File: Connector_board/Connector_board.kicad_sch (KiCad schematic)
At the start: 6 parts, among them J1 USB_B_Micro, J2 Conn_02x04_Counter_Clockwise, J3 Conn_02x06_Counter_Clockwise, J4 Conn_02x07_Counter_Clockwise

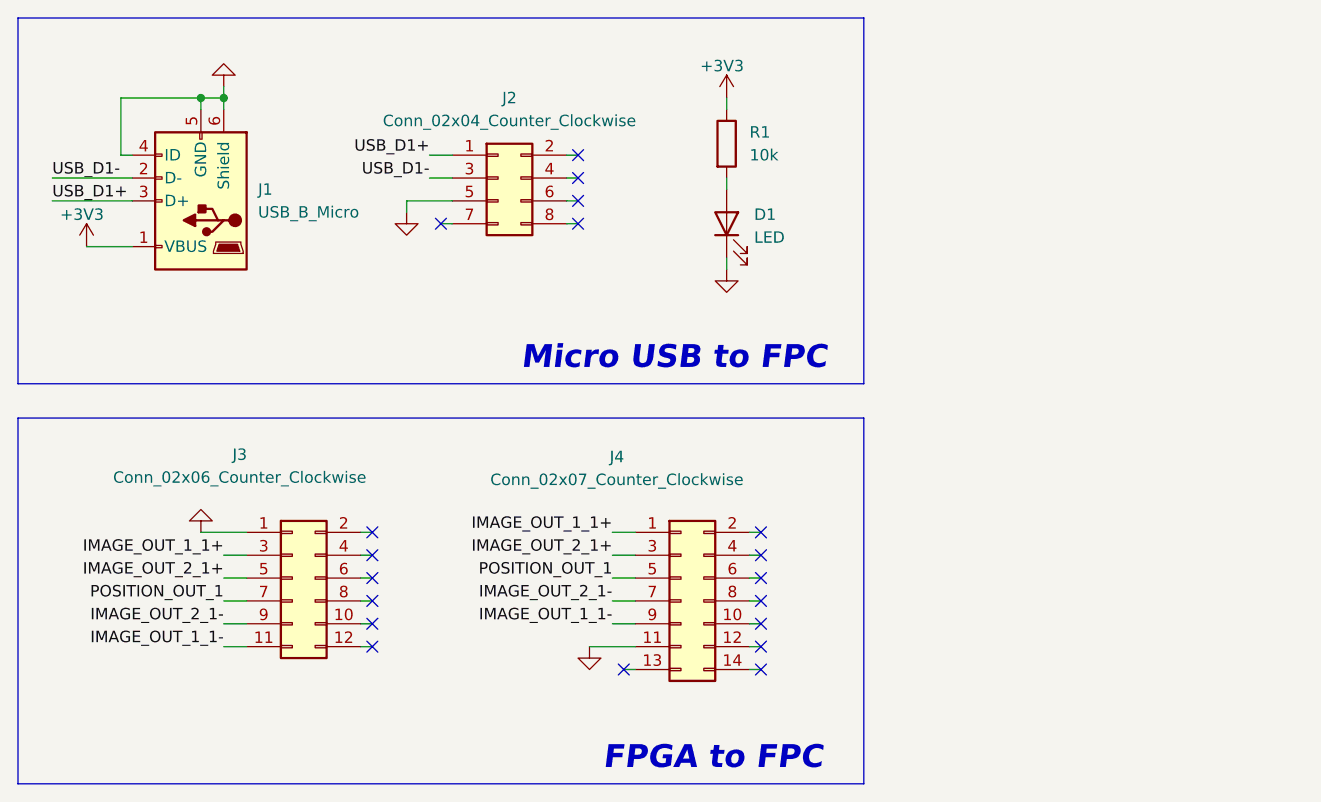
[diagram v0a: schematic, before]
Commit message: layout finalized (?)
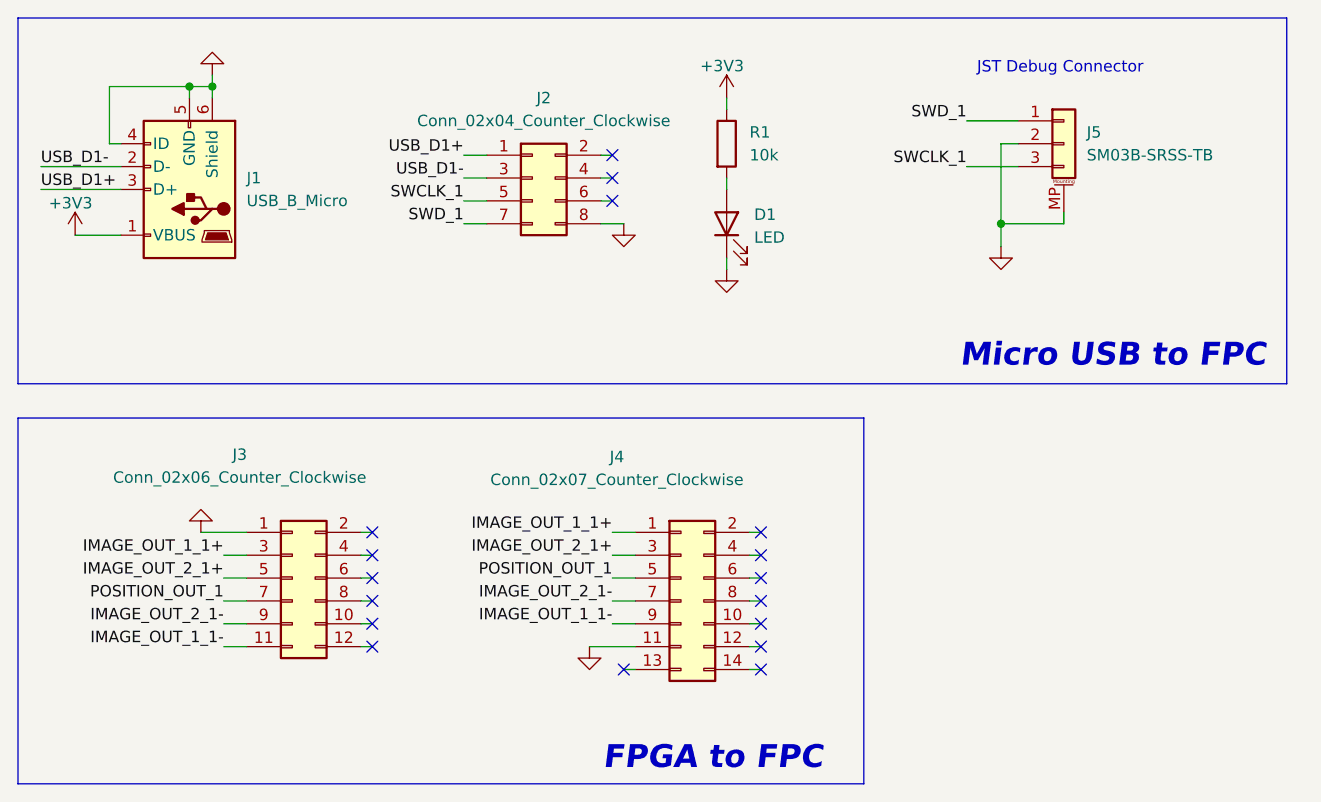
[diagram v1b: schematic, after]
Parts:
- added J5: SM03B-SRSS-TB, Connector_JST:JST_SH_SM03B-SRSS-TB_1x03-1MP_P1.00mm_Horizontal, symbol Connector_Generic_MountingPin:Conn_01x03_MountingPin
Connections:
- net GND: now also J2.8 (Pin_8), J5.2 (Pin_2), J5.MP (MountPin); no longer J2.5 (Pin_5)
- net SWD_1: now reaches J2.7 (Pin_7)
- net SWD_1: now also J5.1 (Pin_1)
- new net SWCLK_1: J2.5 (Pin_5), J5.3 (Pin_3)
- no-connect marks 19 -> 17
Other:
- note added: "JST Debug Connector"
- moved on the sheet: J1, J2
